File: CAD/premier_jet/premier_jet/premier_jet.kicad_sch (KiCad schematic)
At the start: 18 parts, among them J1 Conn_01x03, J2 Conn_01x04, J3 Conn_01x04, J4 Conn_01x04, J5 Barrel_Jack_MountingPin, U4 STM32G474RETx, U5 BU33SD5WG-TR

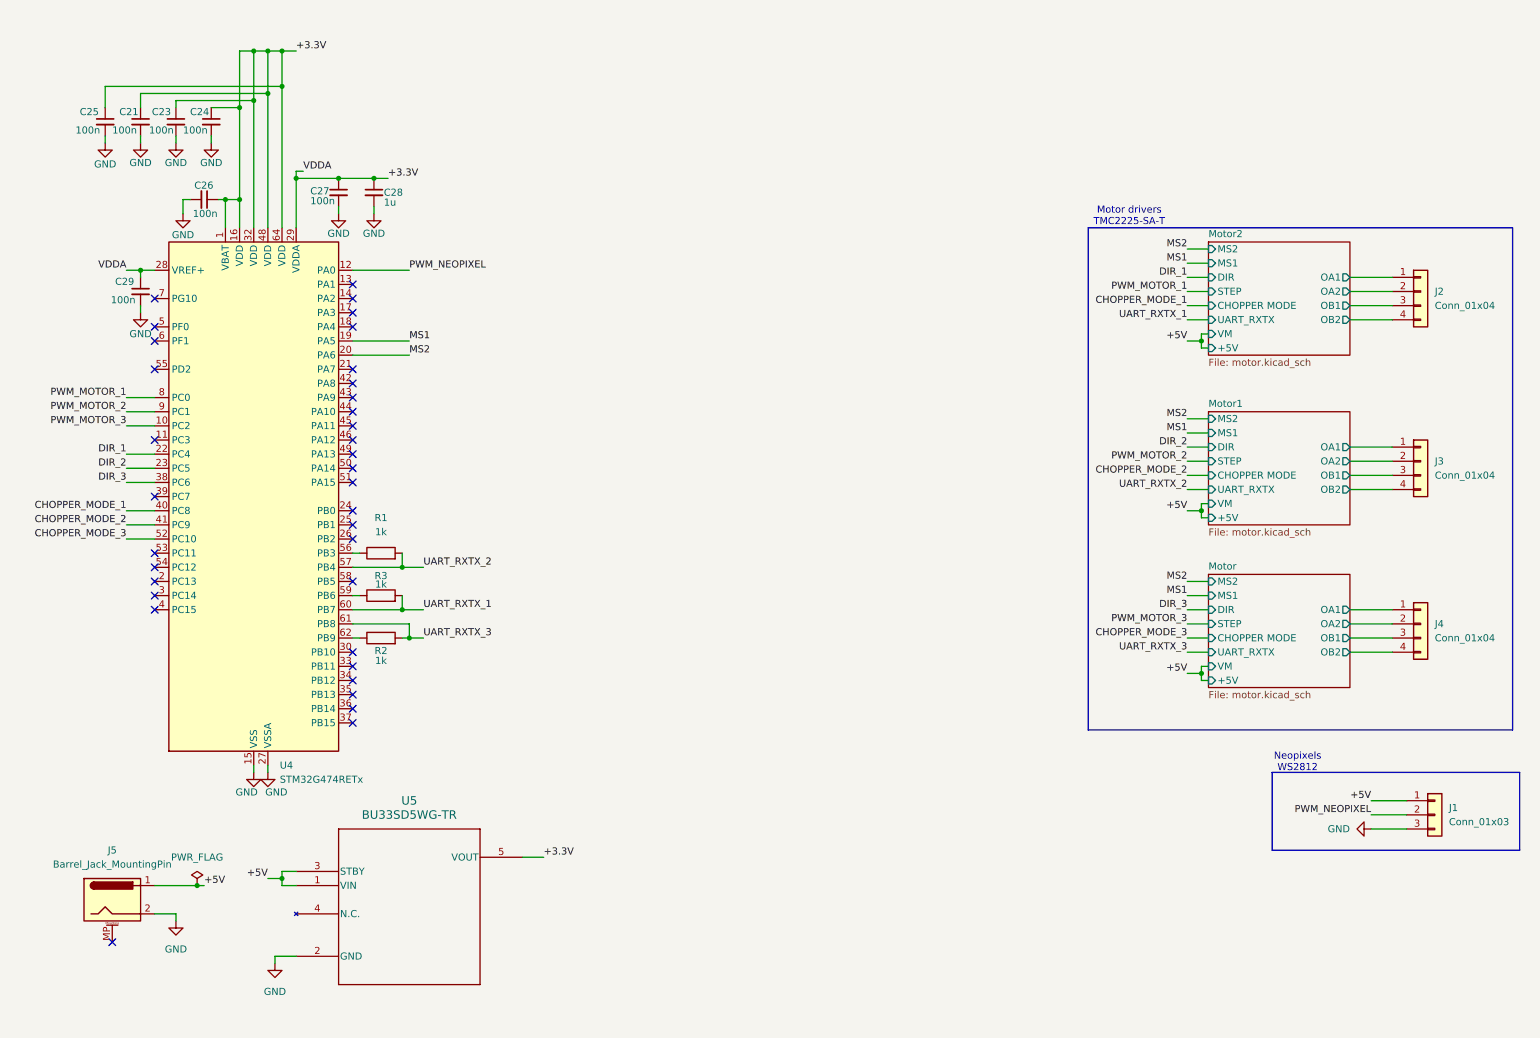
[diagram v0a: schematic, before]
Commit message: Update pcb
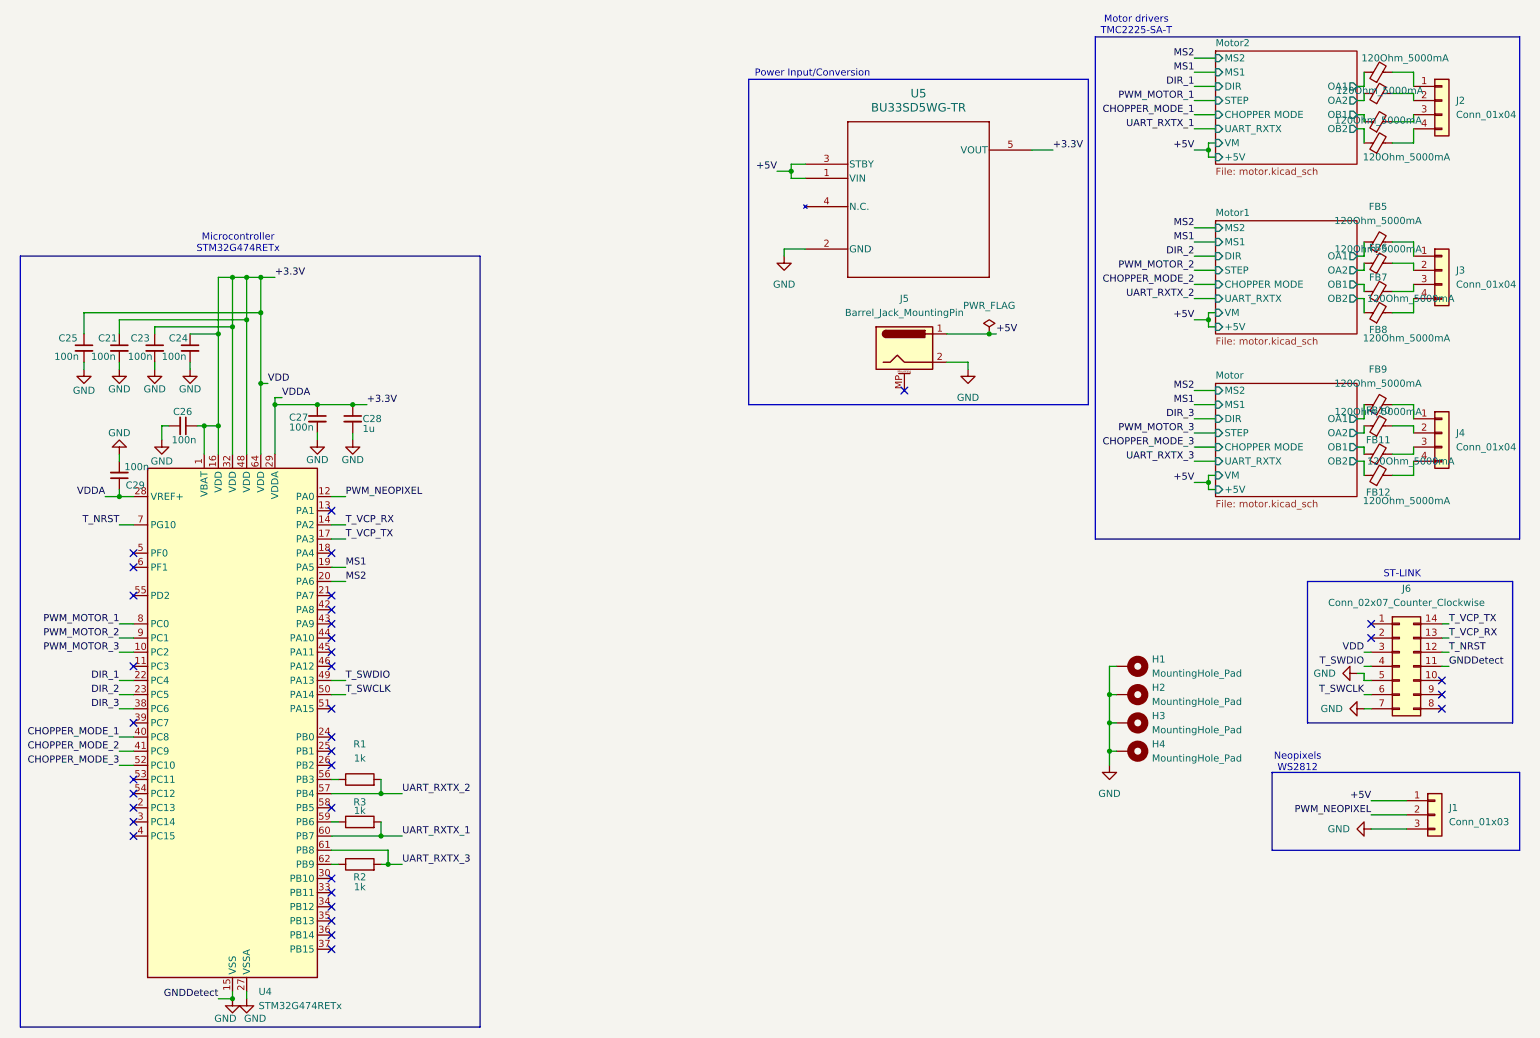
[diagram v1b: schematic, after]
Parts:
- added FB1, FB10, FB11, FB12, FB2, FB3, FB4, FB5, FB6, FB7, FB8, FB9: 120Ohm_5000mA, Inductor_SMD:L_0805_2012Metric, symbol Device:FerriteBead_Small
- added H1, H2, H3, H4: MountingHole_Pad, MountingHole:MountingHole_3.2mm_M3_Pad, symbol Mechanical:MountingHole_Pad
- added J6: Conn_02x07_Counter_Clockwise, Connector_PinHeader_2.54mm:PinHeader_2x07_P2.54mm_Vertical, symbol Connector_Generic:Conn_02x07_Counter_Clockwise
- C21, C23, C24, C25, C26, C27, C28, C29: footprint (none) -> Capacitor_SMD:C_0402_1005Metric
- J1: footprint (none) -> Connector_PinHeader_2.54mm:PinHeader_1x03_P2.54mm_Vertical
- J2, J3, J4: footprint (none) -> Connector_PinHeader_2.54mm:PinHeader_1x04_P2.54mm_Vertical
- R1, R2, R3: footprint (none) -> Resistor_SMD:R_0402_1005Metric
- U5: footprint SSOP5_ROM -> (none)
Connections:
- net +3.3V: now also J6.3 (Pin_3)
- net GND: now also H1.1, H2.1, H3.1, H4.1, J6.11 (Pin_11), J6.5 (Pin_5), J6.7 (Pin_7)
- net Motor/OA1: now also FB9.1; no longer J4.1 (Pin_1)
- net Motor/OA2: now also FB10.1; no longer J4.2 (Pin_2)
- net Motor/OB1: now also FB11.1; no longer J4.3 (Pin_3)
- net Motor/OB2: now also FB12.1; no longer J4.4 (Pin_4)
- net Motor1/OA1: now also FB5.1; no longer J3.1 (Pin_1)
- net Motor1/OA2: now also FB6.1; no longer J3.2 (Pin_2)
- net Motor1/OB1: now also FB7.1; no longer J3.3 (Pin_3)
- net Motor1/OB2: now also FB8.1; no longer J3.4 (Pin_4)
- net Motor2/OA1: now also FB1.1; no longer J2.1 (Pin_1)
- net Motor2/OA2: now also FB2.1; no longer J2.2 (Pin_2)
- net Motor2/OB1: now also FB3.1; no longer J2.3 (Pin_3)
- net Motor2/OB2: now also FB4.1; no longer J2.4 (Pin_4)
- net T_VCP_RX: now reaches U4.14 (PA2)
- net T_VCP_RX: now also J6.13 (Pin_13)
- net T_VCP_TX: now reaches U4.17 (PA3)
- net T_VCP_TX: now also J6.14 (Pin_14)
- net T_SWDIO: now reaches U4.49 (PA13)
- net T_SWDIO: now also J6.4 (Pin_4)
- net T_SWCLK: now reaches U4.50 (PA14)
- net T_SWCLK: now also J6.6 (Pin_6)
- net T_NRST: now reaches U4.7 (PG10)
- net T_NRST: now also J6.12 (Pin_12)
- new net: FB5.2, J3.1 (Pin_1)
- new net: FB1.2, J2.1 (Pin_1)
- new net: FB2.2, J2.2 (Pin_2)
- new net: FB3.2, J2.3 (Pin_3)
- new net: FB4.2, J2.4 (Pin_4)
- new net: FB11.2, J4.3 (Pin_3)
- new net: FB7.2, J3.3 (Pin_3)
- new net: FB9.2, J4.1 (Pin_1)
- new net: FB10.2, J4.2 (Pin_2)
- new net: FB12.2, J4.4 (Pin_4)
- new net: FB6.2, J3.2 (Pin_2)
- new net: FB8.2, J3.4 (Pin_4)
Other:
- note added: "Microcontroller STM32G474RETx"
- note added: "Power Input/Conversion"
- note added: "ST-LINK"
- moved on the sheet: C21, C23, C24, C25, C26, C27, C28, C29, J2, J3, J4, J5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
